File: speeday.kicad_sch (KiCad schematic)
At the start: 1 part, among them U1 STM32F107V_B-C_Tx

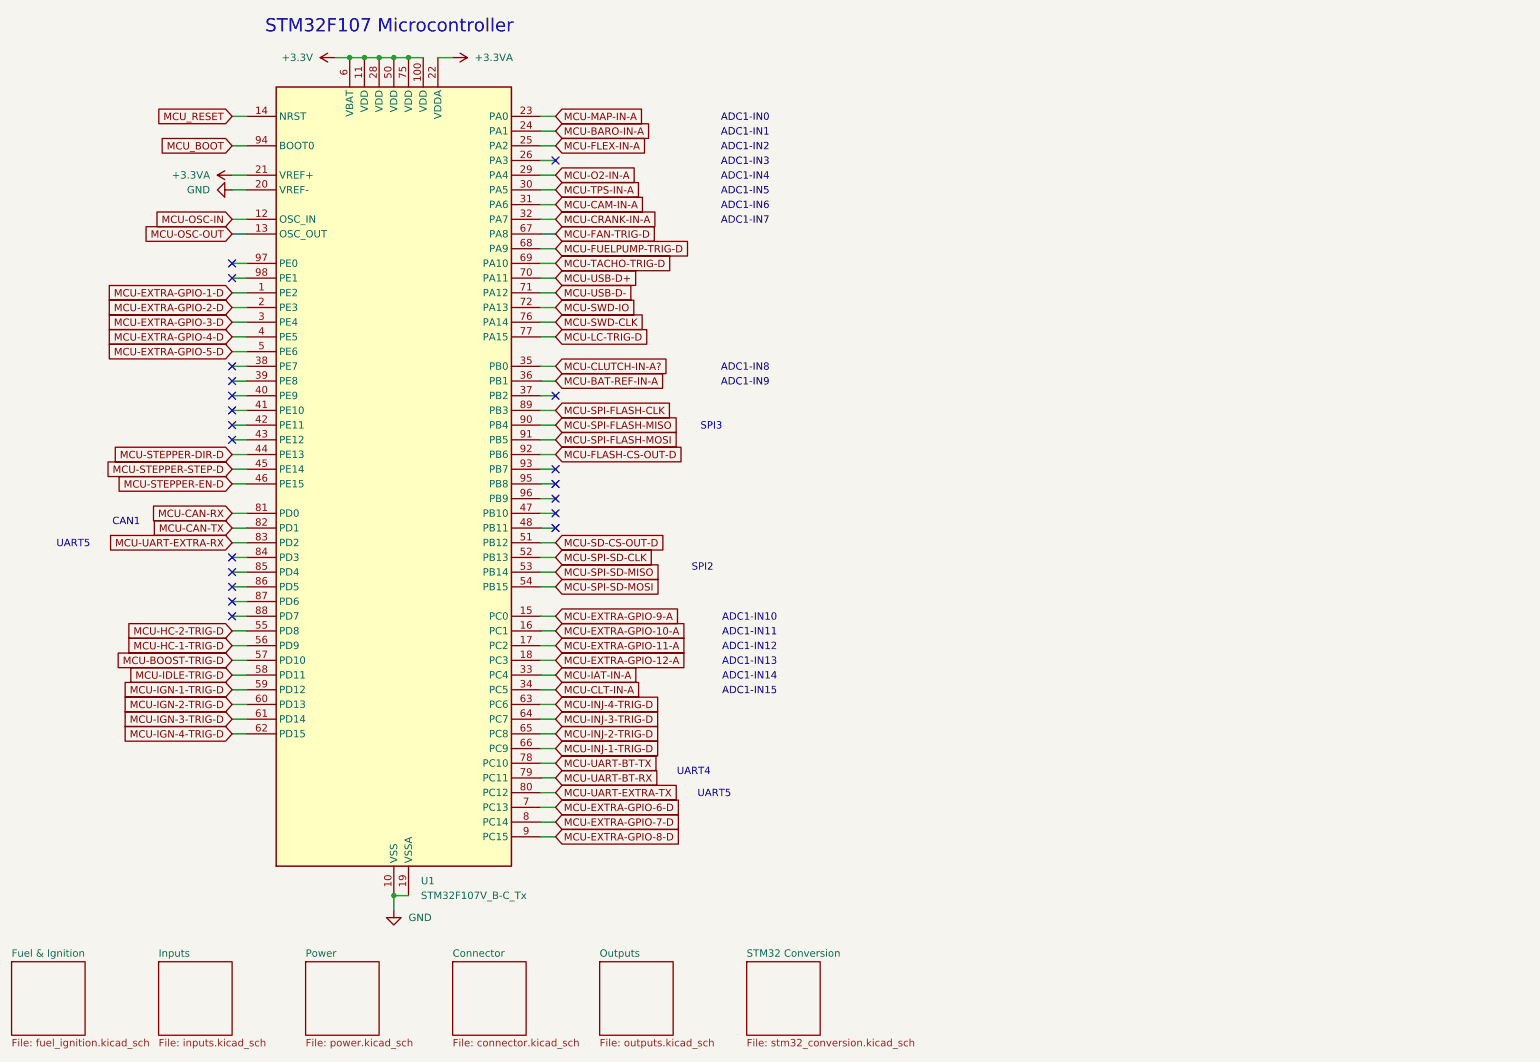
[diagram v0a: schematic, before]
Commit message: Pre MCU switch
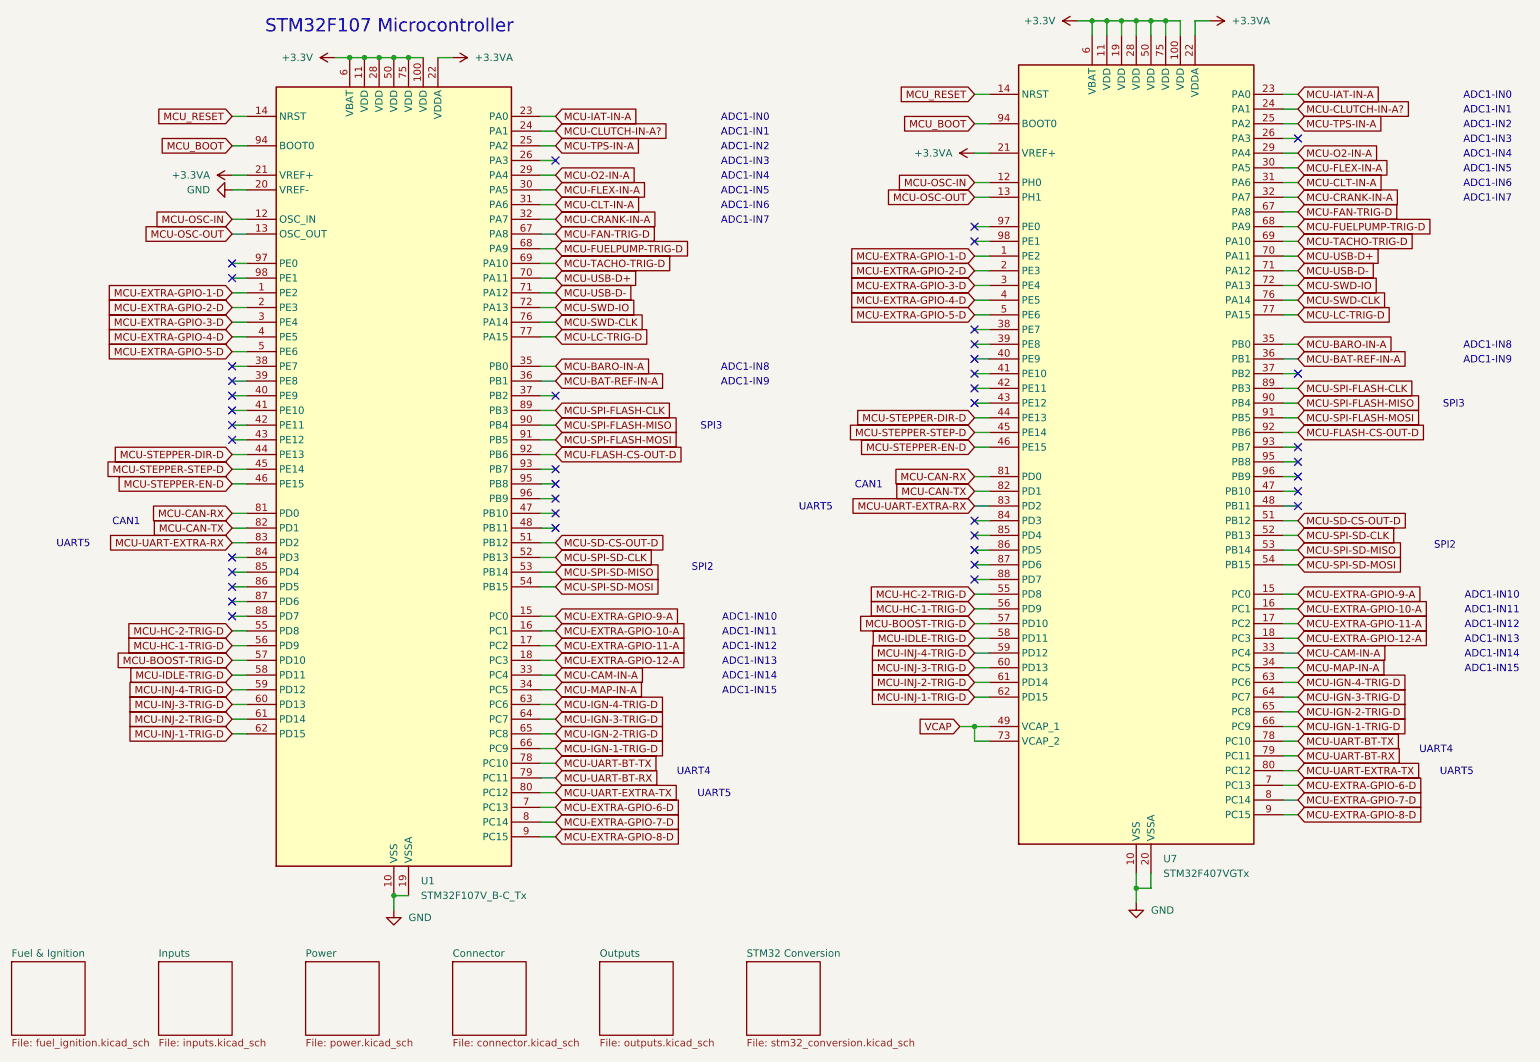
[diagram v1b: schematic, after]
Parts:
- added U7: STM32F407VGTx, Package_QFP:LQFP-176_24x24mm_P0.5mm, symbol MCU_ST_STM32F4:STM32F407VGTx
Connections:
- net +3.3V: now also U7.100 (VDD), U7.11 (VDD), U7.19 (VDD), U7.28 (VDD), U7.50 (VDD), U7.6 (VBAT), U7.75 (VDD)
- net +3.3VA: now also U7.21 (VREF+), U7.22 (VDDA)
- net GND: now also U7.10 (VSS), U7.20 (VSSA), U7.27 (VSS), U7.74 (VSS), U7.99 (VSS)
- net MCU-BARO-IN-A: now also U1.35 (PB0), U7.35 (PB0); no longer U1.24 (PA1)
- net MCU-BAT-REF-IN-A: now also U7.36 (PB1)
- net MCU-BOOST-TRIG-D: now also U7.57 (PD10)
- net MCU-CAM-IN-A: now also U1.33 (PC4), U7.33 (PC4); no longer U1.31 (PA6)
- net MCU-CAN-RX: now also U7.81 (PD0)
- net MCU-CAN-TX: now also U7.82 (PD1)
- net MCU-CLT-IN-A: now also U1.31 (PA6), U7.31 (PA6); no longer U1.34 (PC5)
- net MCU-CLUTCH-IN-A?: now also U1.24 (PA1), U7.24 (PA1); no longer U1.35 (PB0)
- net MCU-CRANK-IN-A: now also U7.32 (PA7)
- net MCU-EXTRA-GPIO-1-D: now also U7.1 (PE2)
- net MCU-EXTRA-GPIO-10-A: now also U7.16 (PC1)
- net MCU-EXTRA-GPIO-11-A: now also U7.17 (PC2)
- net MCU-EXTRA-GPIO-12-A: now also U7.18 (PC3)
- net MCU-EXTRA-GPIO-2-D: now also U7.2 (PE3)
- net MCU-EXTRA-GPIO-3-D: now also U7.3 (PE4)
- net MCU-EXTRA-GPIO-4-D: now also U7.4 (PE5)
- net MCU-EXTRA-GPIO-5-D: now also U7.5 (PE6)
- net MCU-EXTRA-GPIO-6-D: now also U7.7 (PC13)
- net MCU-EXTRA-GPIO-7-D: now also U7.8 (PC14)
- net MCU-EXTRA-GPIO-8-D: now also U7.9 (PC15)
- net MCU-EXTRA-GPIO-9-A: now also U7.15 (PC0)
- net MCU-FAN-TRIG-D: now also U7.67 (PA8)
- net MCU-FLASH-CS-OUT-D: now also U7.92 (PB6)
- net MCU-FLEX-IN-A: now also U1.30 (PA5), U7.30 (PA5); no longer U1.25 (PA2)
- net MCU-FUELPUMP-TRIG-D: now also U7.68 (PA9)
- net MCU-HC-1-TRIG-D: now also U7.56 (PD9)
- net MCU-HC-2-TRIG-D: now also U7.55 (PD8)
- net MCU-IAT-IN-A: now also U1.23 (PA0), U7.23 (PA0); no longer U1.33 (PC4)
- net MCU-IDLE-TRIG-D: now also U7.58 (PD11)
- net MCU-IGN-1-TRIG-D: now also U1.66 (PC9), U7.66 (PC9); no longer U1.59 (PD12)
- net MCU-IGN-2-TRIG-D: now also U1.65 (PC8), U7.65 (PC8); no longer U1.60 (PD13)
- net MCU-IGN-3-TRIG-D: now also U1.64 (PC7), U7.64 (PC7); no longer U1.61 (PD14)
- net MCU-IGN-4-TRIG-D: now also U1.63 (PC6), U7.63 (PC6); no longer U1.62 (PD15)
- net MCU-INJ-1-TRIG-D: now also U1.62 (PD15), U7.62 (PD15); no longer U1.66 (PC9)
- net MCU-INJ-2-TRIG-D: now also U1.61 (PD14), U7.61 (PD14); no longer U1.65 (PC8)
- net MCU-INJ-3-TRIG-D: now also U1.60 (PD13), U7.60 (PD13); no longer U1.64 (PC7)
- net MCU-INJ-4-TRIG-D: now also U1.59 (PD12), U7.59 (PD12); no longer U1.63 (PC6)
- net MCU-LC-TRIG-D: now also U7.77 (PA15)
- net MCU-MAP-IN-A: now also U1.34 (PC5), U7.34 (PC5); no longer U1.23 (PA0)
- net MCU-O2-IN-A: now also U7.29 (PA4)
- net MCU-OSC-IN: now also U7.12 (PH0)
- net MCU-OSC-OUT: now also U7.13 (PH1)
- net MCU-SD-CS-OUT-D: now also U7.51 (PB12)
- net MCU-SPI-FLASH-CLK: now also U7.89 (PB3)
- net MCU-SPI-FLASH-MISO: now also U7.90 (PB4)
- net MCU-SPI-FLASH-MOSI: now also U7.91 (PB5)
- net MCU-SPI-SD-CLK: now also U7.52 (PB13)
- net MCU-SPI-SD-MISO: now also U7.53 (PB14)
- net MCU-SPI-SD-MOSI: now also U7.54 (PB15)
- net MCU-STEPPER-DIR-D: now also U7.44 (PE13)
- net MCU-STEPPER-EN-D: now also U7.46 (PE15)
- net MCU-STEPPER-STEP-D: now also U7.45 (PE14)
- net MCU-SWD-CLK: now also U7.76 (PA14)
- net MCU-SWD-IO: now also U7.72 (PA13)
- net MCU-TACHO-TRIG-D: now also U7.69 (PA10)
- net MCU-TPS-IN-A: now also U1.25 (PA2), U7.25 (PA2); no longer U1.30 (PA5)
- net MCU-UART-BT-RX: now also U7.79 (PC11)
- net MCU-UART-BT-TX: now also U7.78 (PC10)
- net MCU-UART-EXTRA-RX: now also U7.83 (PD2)
- net MCU-UART-EXTRA-TX: now also U7.80 (PC12)
- net MCU-USB-D+: now also U7.70 (PA11)
- net MCU-USB-D-: now also U7.71 (PA12)
- net MCU_BOOT: now also U7.94 (BOOT0)
- net MCU_RESET: now also U7.14 (NRST)
- new net VCAP: U7.49 (VCAP_1), U7.73 (VCAP_2)
- no-connect marks 20 -> 40
